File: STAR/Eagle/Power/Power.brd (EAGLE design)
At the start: 66 x 44.5 mm, 24 parts, among them J1 J30J-9J30, T1 750311838, U1 LT8300, U2 LT8330

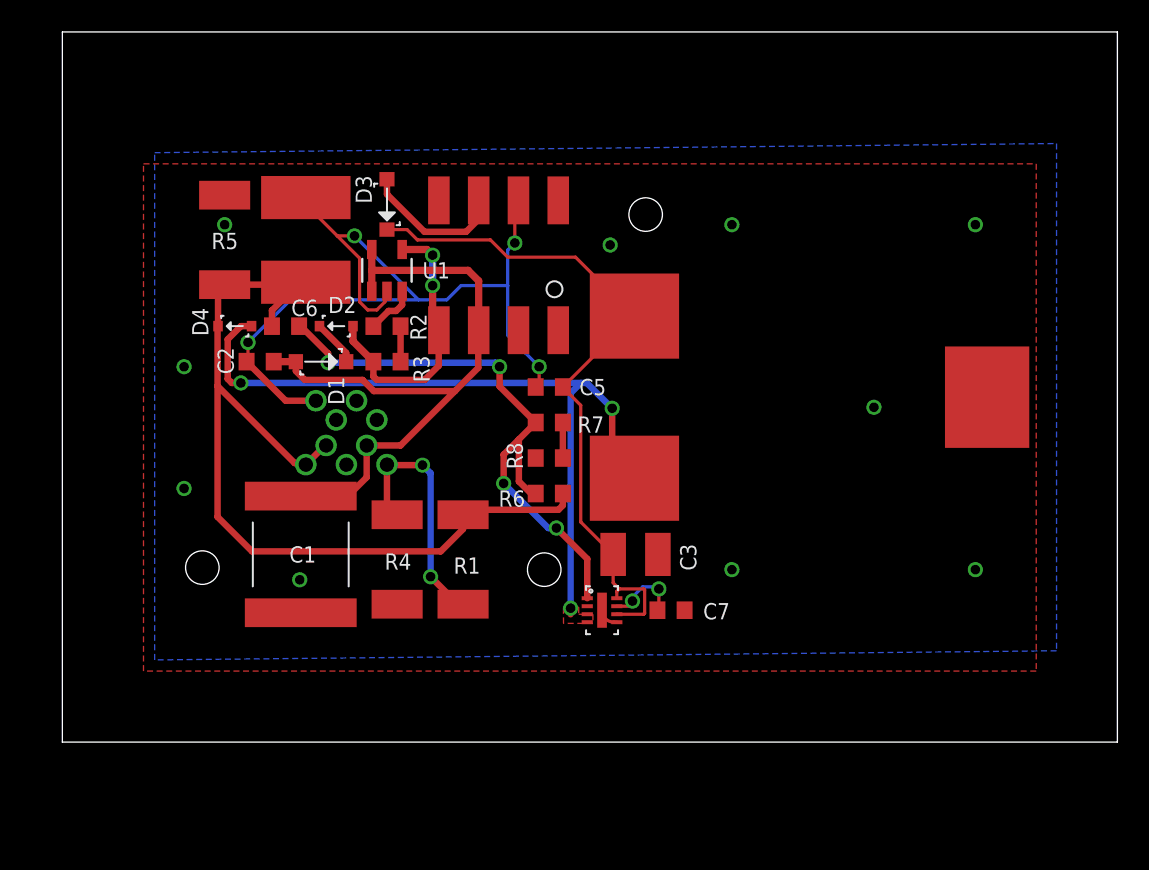
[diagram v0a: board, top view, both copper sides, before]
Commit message: Power Board
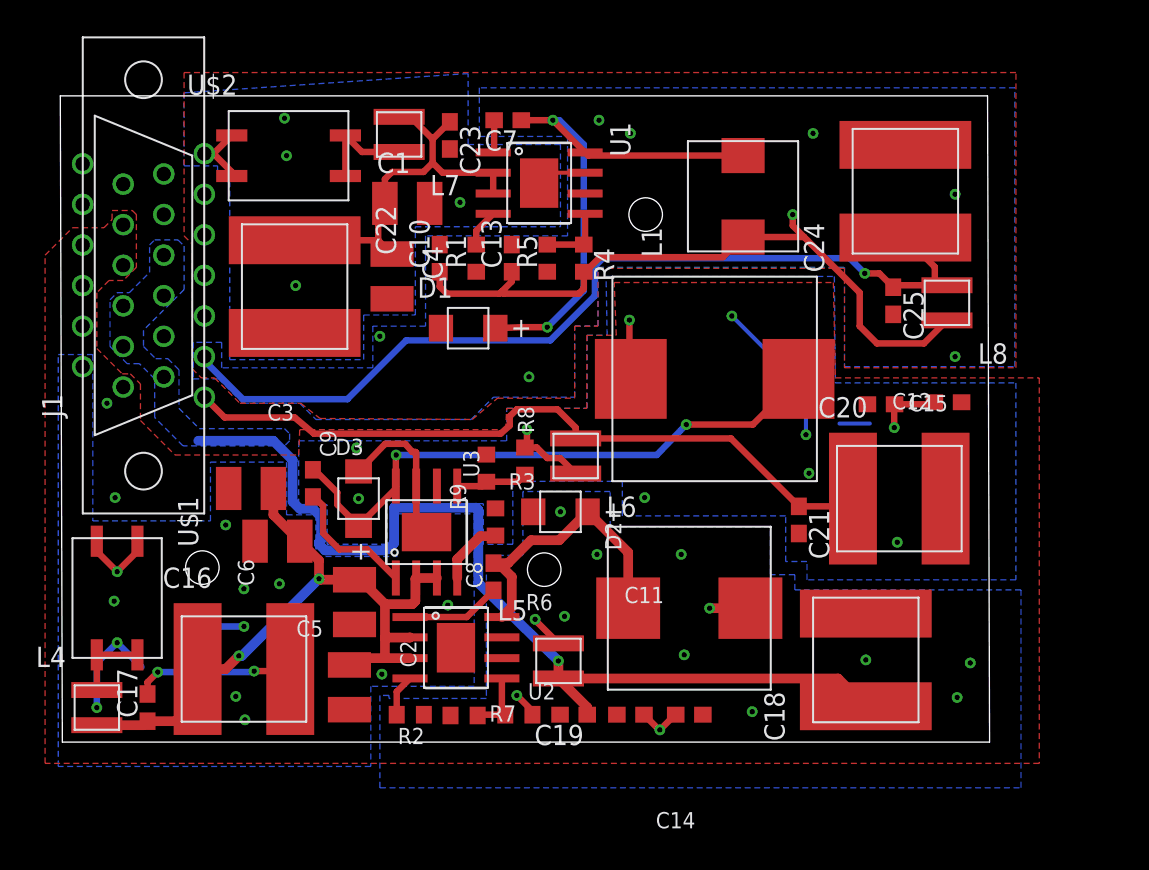
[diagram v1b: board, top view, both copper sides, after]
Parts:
- removed D4: PMEG6010CEJ, AR_diode:SOD323
- removed T1: 750311838, AR_transformer:750311838
- added C10, C11, C12: .18 uF, resistor:C0603
- added C13, C14, C15: 10 uF, resistor:C0603
- added C16, C18, C20, C22, C24: KTJ500B476M76BFT00, Filtering:STACKED
- added C17, C19, C21, C23, C25: 1nF, resistor:C0603
- added C8, C9: .1 uF, resistor:C0603
- added L2: 5.5u, Filtering:1050
- added L3: 3.7u, Power:1365
- added L4, L5, L6, L7, L8: 744029000068, Filtering:2813
- added R9: 13.3k, resistor:R0603
- added U$1, U$2: DFT7160-105B, Filtering:DFT7160
- added U3: LMR16020, HASP:SO8
- C1: value 22uF -> 10 uF; device AR_passives:3025 -> resistor:C1210
- C2: value 1uF -> 10 uF; device AR_passives:0603 -> resistor:C1210
- C3: value (none) -> 10 uF
- C4: value 10uF -> 2.2 uF; device AR_passives:2J-LEAD -> resistor:C1210
- C5: value 1uF -> 2.2 uF; device AR_passives:0603 -> resistor:C1210
- C6: value 4.7pF -> 2.2 uF; device AR_passives:0603 -> resistor:C1210
- C7: value 1uF -> .1 uF; device AR_passives:0603 -> resistor:C0603
- D1: value MMSZ5266BT1G -> DO-214AC; device AR_diode:SOD123 -> HASP:DO-214AC
- D2: value BAV20W -> DO-214AC; device AR_diode:SOD323 -> HASP:DO-214AC
- D3: value SBR0560S1 -> DO-214AC; device AR_diode:SOD123 -> HASP:DO-214AC
- J1: value J30J-9J30 -> J30J-25; device CM_J30J:ZKN-9-J30 -> CM_J30J:ZKN-25
- L1: value 10uH -> 9.7u; device AR_passives:PQ2614 -> Power:7050
- R1: value 47k -> 23.2k; device resistor:R2512 -> resistor:R0603
- R2: value 407k -> 23.2k
- R3: value 1k -> 23.2k
- R4: value 3k -> 199.5k; device resistor:R2512 -> resistor:R0603
- R5: value 1.5k -> 13.3k; device resistor:R2512 -> resistor:R0603
- R6: value 1M -> 75.4k
- R7: value 33k -> 13.3k
- R8: value 52.6 -> 45.2k
- U1: value LT8300 -> LMR16020; device AR_IC:SOT23-5 -> HASP:SO8
- U2: value LT8330 -> LMR16020; device AR_IC:8-DFN -> HASP:SO8
- moved C7 32.3 mm to (21.5, 32.6), turned to 180 degrees
- moved C3 24.4 mm to (5.46, 9.53), turned to 180 degrees
- moved R2 24.4 mm to (15.4, -4.64), turned to 180 degrees
- moved C1 23.0 mm to (15.2, 27.4), turned to 0 degrees
- moved R4 22.2 mm to (26.3, 23.9), turned to 270 degrees
- moved C2 21.1 mm to (11.6, -2.92), turned to 270 degrees
- moved R5 20.2 mm to (24.0, 23.9), turned to 90 degrees
- moved C5 19.6 mm to (7.11, 6.22)
- moved R7 19.1 mm to (18.8, -4.69), turned to 0 degrees
- moved R1 18.9 mm to (19.6, 23.9)
- moved D3 18.5 mm to (12.2, 8.89)
- moved D2 18.2 mm to (24.8, 8.06), turned to 0 degrees
- moved C6 17.8 mm to (11.9, 2.41), turned to 270 degrees
- moved J1 16.1 mm to (-1.27, 22.9), turned to 90 degrees
- moved L1 14.7 mm to (36.3, 27.8), turned to 90 degrees
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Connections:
- removed net +20V: C3.1, C5.1, D3.P$2, L1.P$2, U2.P$6, U2.P$8
- removed net +50V: C4.P$1, C6.1, D4.P$2, J1.1, J1.2, R1.2, R5.2, R6.2
- removed net N$11: R7.1, R8.2
- removed net VCC: C1.P$1, C2.1, D1.P$1, J1.4, T1.P$3, U1.1, U1.5
- removed net V_DIVIDE: J1.5, R1.1, R4.2
- new net +12V: C10.1, C13.1, L1.P$2, L8.P$1, R4.2
- new net +3V3: C12.1, C15.1, L3.P$2, L6.P$1, R8.2
- new net +5V: C11.1, C14.1, L2.P$2, L5.P$1, R6.2
- new net 12V_FILT: C24.P$1, C25.1, J1.3, L8.P$2
- new net 3V3_FILT: C20.P$1, C21.1, J1.1, L6.P$2
- new net 5V_FILT: C18.P$1, C19.1, J1.16, J1.18, J1.2, J1.8, L5.P$2
- new net D: J1.10
- new net ER: J1.12
- new net F: J1.6
- new net GSE_FILT: C16.P$1, C17.1, C2.1, C3.1, C5.1, C6.1, L4.P$2, U2.P$2, U2.P$3, U3.P$2, U3.P$3
- new net GSE_GND: C11.2, C12.2, C14.2, C15.2, C16.P$2, C17.2, C18.P$2, C19.2, C2.2, C20.P$2, C21.2, C3.2, C5.2, C6.2, D2.P$1, D3.P$1, J1.14, J1.17, J1.19, J1.20, J1.21, J1.22, R2.1, R3.1, R7.1, R9.1, U2.P$7, U2.PAD, U3.P$7, U3.PAD
- new net GSE_UFILT: J1.15, U$1.P$1, U$1.P$2
- new net I: J1.4
- new net N$14: C7.1, D1.P$2, L1.P$1, U1.P$8
- new net N$27: R4.1, R5.2, U1.P$5
- new net N$28: L4.P$1, U$1.P$3, U$1.P$4
- new net N$29: L7.P$1, U$2.P$3, U$2.P$4
- new net N$44: J1.25
- new net N$45: J1.24
- new net N$46: J1.23
- new net N$8: R8.1, R9.2, U3.P$5
- new net Q: J1.7
- new net T: J1.5
- new net TE_FILT: C1.1, C22.P$1, C23.1, C4.1, L7.P$2, U1.P$2, U1.P$3
- new net TE_UFILT: J1.13, U$2.P$1, U$2.P$2
- net GND: now also C1.2, C10.2, C13.2, C22.P$2, C23.2, C24.P$2, C25.2, C4.2, D1.P$1, J1.11, J1.9, R1.1, U1.P$7, U1.PAD; no longer C1.P$2, C2.2, C3.2, C4.P$2, C5.2, C7.2, J1.6, J1.7, R4.1, R8.1, T1.P$7, U1.2, U2.P$5, U2.P$9
- net N$1: now also R3.2, U3.P$4; no longer D1.P$2, D2.P$2
- net N$10: now also C7.2, U1.P$1; no longer J1.9
- net N$2: now also C9.1, D3.P$2, L3.P$1, U3.P$8; no longer R2.1, U1.3
- net N$3: now also U2.P$4; no longer R3.1
- net N$4: now also C8.2, U2.P$1; no longer D2.P$1, R3.2, T1.P$4, U1.4
- net N$5: now also C8.1, D2.P$2, L2.P$1, U2.P$8; no longer D3.P$1, T1.P$6
- net N$6: now also C9.2, U3.P$1; no longer C7.1, U2.P$7
- net N$7: now also R1.2, U1.P$4; no longer D4.P$1, L1.P$3, U2.P$3, U2.P$4
- net N$9: now also U2.P$5; no longer C6.2, U2.P$1
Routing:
- net 5V_FILT: track 0.00 -> 61.2 mm, vias 0 -> 1
- net +50V: track 57.6 -> 0.00 mm
- net 12V_FILT: track 0.00 -> 57.0 mm, vias 0 -> 1
- net GND: track 55.8 -> 3.14 mm, vias 14 -> 6
- net N$7: track 48.8 -> 2.37 mm, vias 3 -> 0
- net 3V3_FILT: track 0.00 -> 45.6 mm
- net GSE_FILT: track 0.00 -> 44.1 mm, vias 0 -> 2
- net +20V: track 43.6 -> 0.00 mm
- net VCC: track 43.1 -> 0.00 mm
- net +12V: track 0.00 -> 42.8 mm, vias 0 -> 3
- net N$2: track 3.21 -> 37.4 mm, vias 0 -> 2
- net GSE_GND: track 0.00 -> 34.1 mm, vias 0 -> 14
- net N$14: track 0.00 -> 33.0 mm, vias 0 -> 2
- net N$9: track 36.7 -> 4.11 mm, vias 4 -> 0
- net TE_FILT: track 0.00 -> 24.9 mm
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- added copper zone on layer 16, net +12V
- added copper zone on layer 16, net +3V3
- added copper zone on layer 16, net +5V
- added copper zone on layer 16, net 5V_FILT
- added copper zone on layer 1, net GSE_GND
- added copper zone on layer 16, net GSE_UFILT
- added copper zone on layer 16, net TE_UFILT
- removed copper zone on layer 16, net GND
- removed copper zone on layer 1, net N$7
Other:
- board size 66 x 44.5 mm -> 58.2 x 40.4 mm
